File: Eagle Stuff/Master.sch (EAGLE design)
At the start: 5 parts

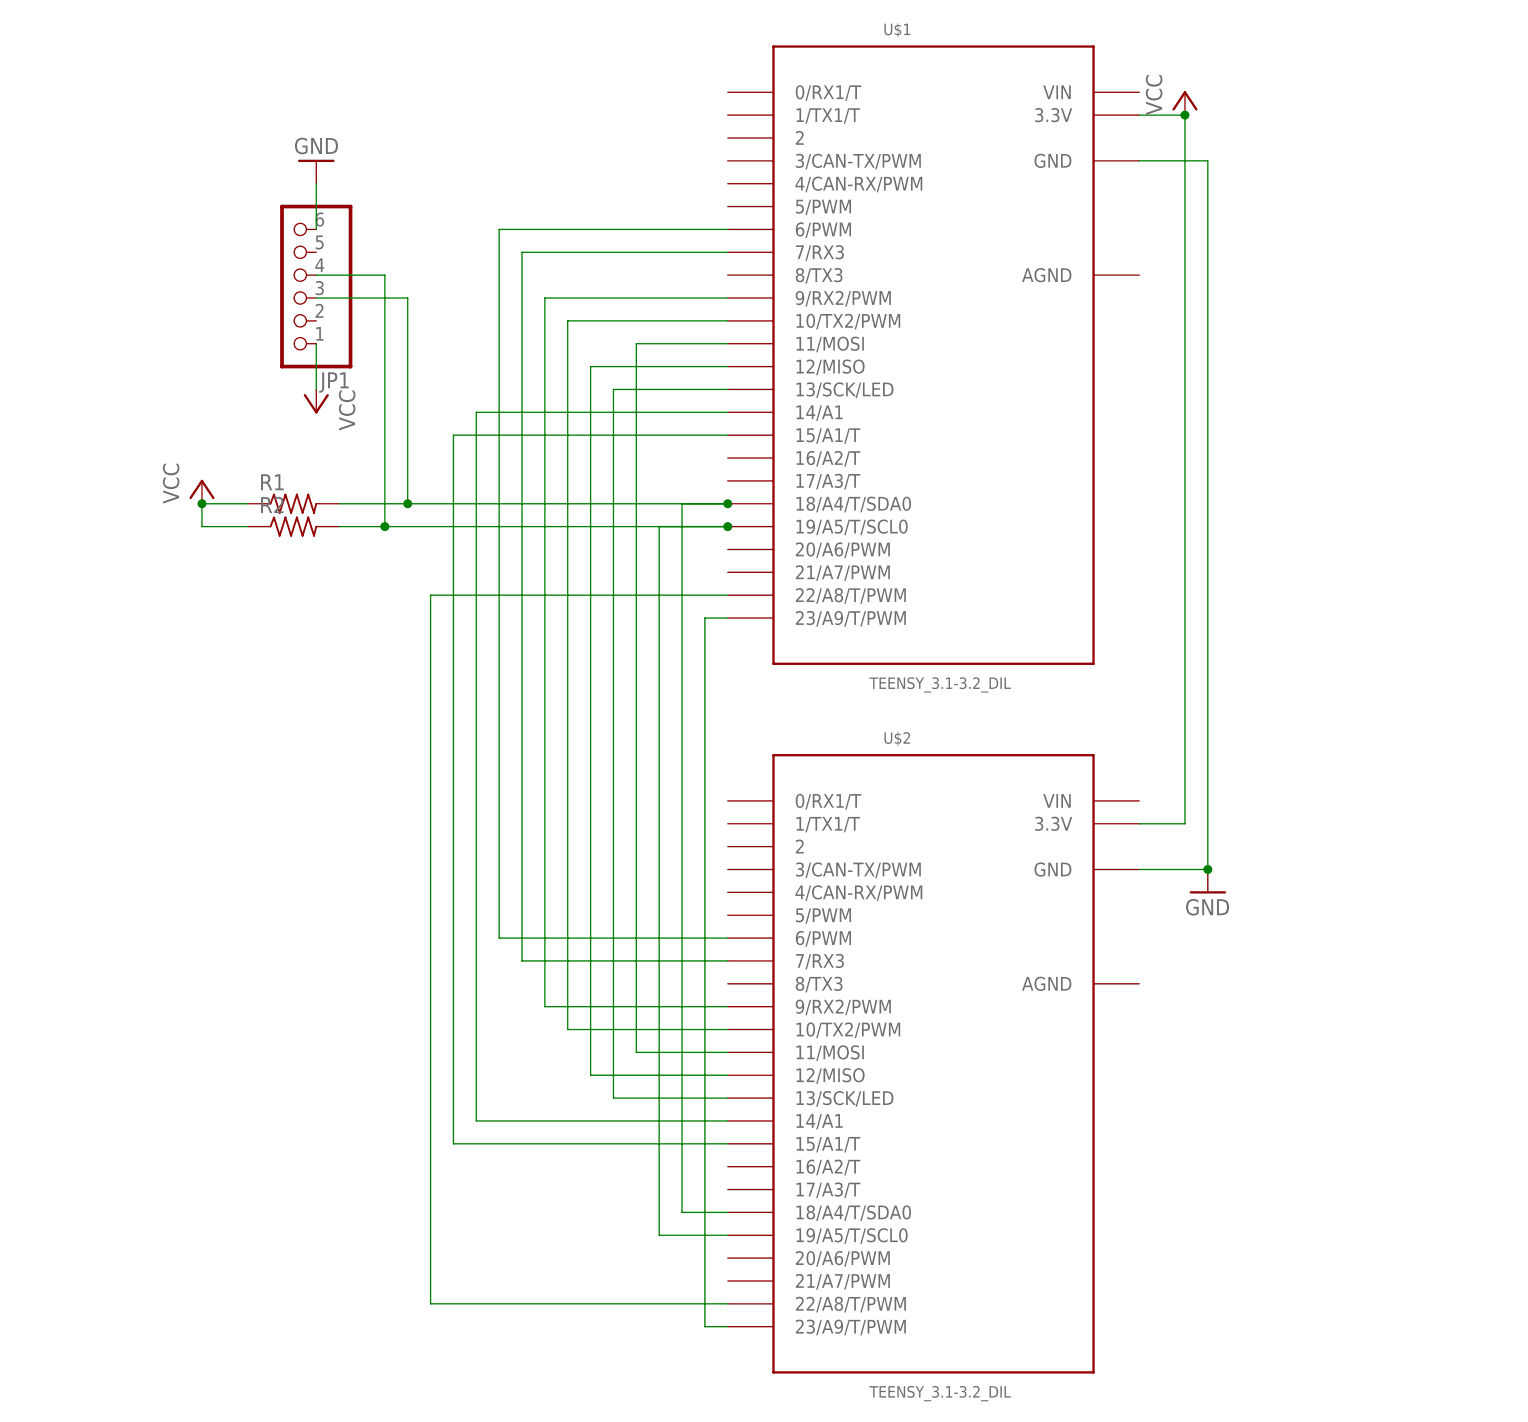
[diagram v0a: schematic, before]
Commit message: Initial commit for master board
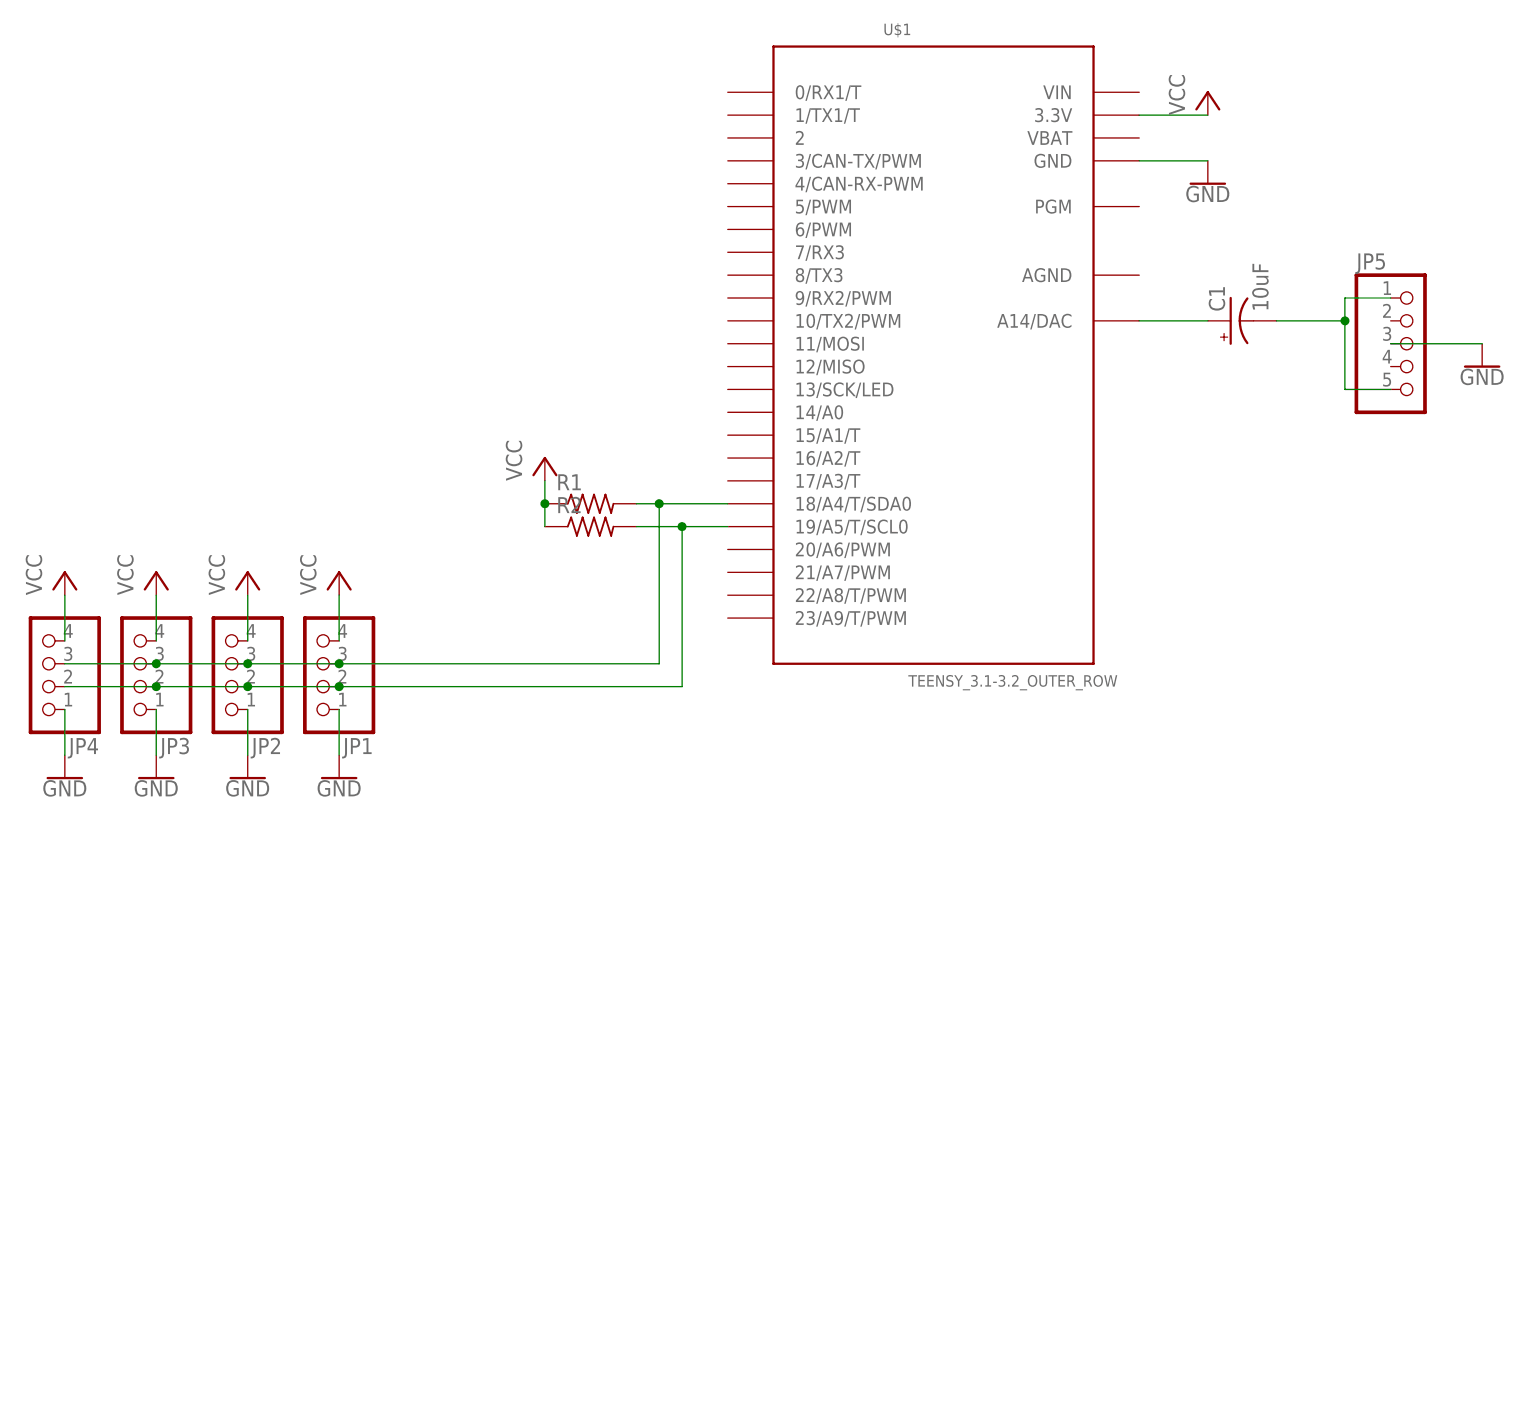
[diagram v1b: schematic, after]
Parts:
- removed U$2: TEENSY_3.1-3.2_DIL, Teensy_3_and_LC_Series_Boards_v1.4:TEENSY_3.1-3.2_DIL
- added C1: 10uF, SparkFun-Capacitors:10UF-POLAR-RADIAL-2.5MM-25V-20%
- added JP2, JP3, JP4: (no value), pinhead:PINHD-1X4
- added JP5: (no value), pinhead:PINHD-1X5
- JP1: device pinhead:PINHD-1X6 -> pinhead:PINHD-1X4
- U$1: value TEENSY_3.1-3.2_DIL -> TEENSY_3.1-3.2_OUTER_ROW; device Teensy_3_and_LC_Series_Boards_v1.4:TEENSY_3.1-3.2_DIL -> Teensy_3_and_LC_Series_Boards_v1.4:TEENSY_3.1-3.2_OUTER_ROW
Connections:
- removed net N$10: U$1.6/PWM, U$2.6/PWM
- removed net N$11: U$1.13/SCK/LED, U$2.13/SCK/LED
- removed net N$12: U$1.14/A1, U$2.14/A1
- removed net N$13: U$1.15/A1/T, U$2.15/A1/T
- removed net N$14: U$1.23/A9/T/PWM, U$2.23/A9/T/PWM
- removed net N$15: U$1.22/A8/T/PWM, U$2.22/A8/T/PWM
- removed net N$5: U$1.11/MOSI, U$2.11/MOSI
- removed net N$6: U$1.12/MISO, U$2.12/MISO
- removed net N$7: U$1.10/TX2/PWM, U$2.10/TX2/PWM
- removed net N$8: U$1.9/RX2/PWM, U$2.9/RX2/PWM
- removed net N$9: U$1.7/RX3, U$2.7/RX3
- new net N$1: JP1.3, JP2.3, JP3.3, JP4.3, R1.2, U$1.18/A4/T/SDA0
- new net N$4: C1.-, JP5.1, JP5.5
- net GND: now also JP1.1, JP2.1, JP3.1, JP4.1, JP5.3; no longer JP1.6, U$2.GND
- net N$2: now also JP1.2, JP2.2, JP3.2, JP4.2, R2.2, U$1.19/A5/T/SCL0; no longer JP1.3, R1.2, U$1.18/A4/T/SDA0, U$2.18/A4/T/SDA0
- net N$3: now also C1.+, U$1.A14/DAC; no longer JP1.4, R2.2, U$1.19/A5/T/SCL0, U$2.19/A5/T/SCL0
- net VCC: now also JP1.4, JP2.4, JP3.4, JP4.4; no longer JP1.1, U$2.3.3V
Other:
- moved on the sheet: R1, R2
